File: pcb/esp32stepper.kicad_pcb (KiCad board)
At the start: 4 copper layers, 40 x 40 mm, 86 parts, among them J1 JTAG, J2 Stepper, J3 Display 0.96" 128x96, J4 IO, J5 Qwiic_Vertical, J6 FAN, J7 PWR, J8 USB_C_Receptacle_USB2.0_14P, Q1 IRLML9301, Q2 IRLML9301, SW1 RST, SW3 BOOT, SW4 B1, SW5 B2, U1 TMC2208-LA, U2 ESP32-S3-MINI-1, U3 MPU-9250, U4 AS5048B, U5 LM555xMM, U6 TPS56339DDC, U7 CH224K, U8 BME280

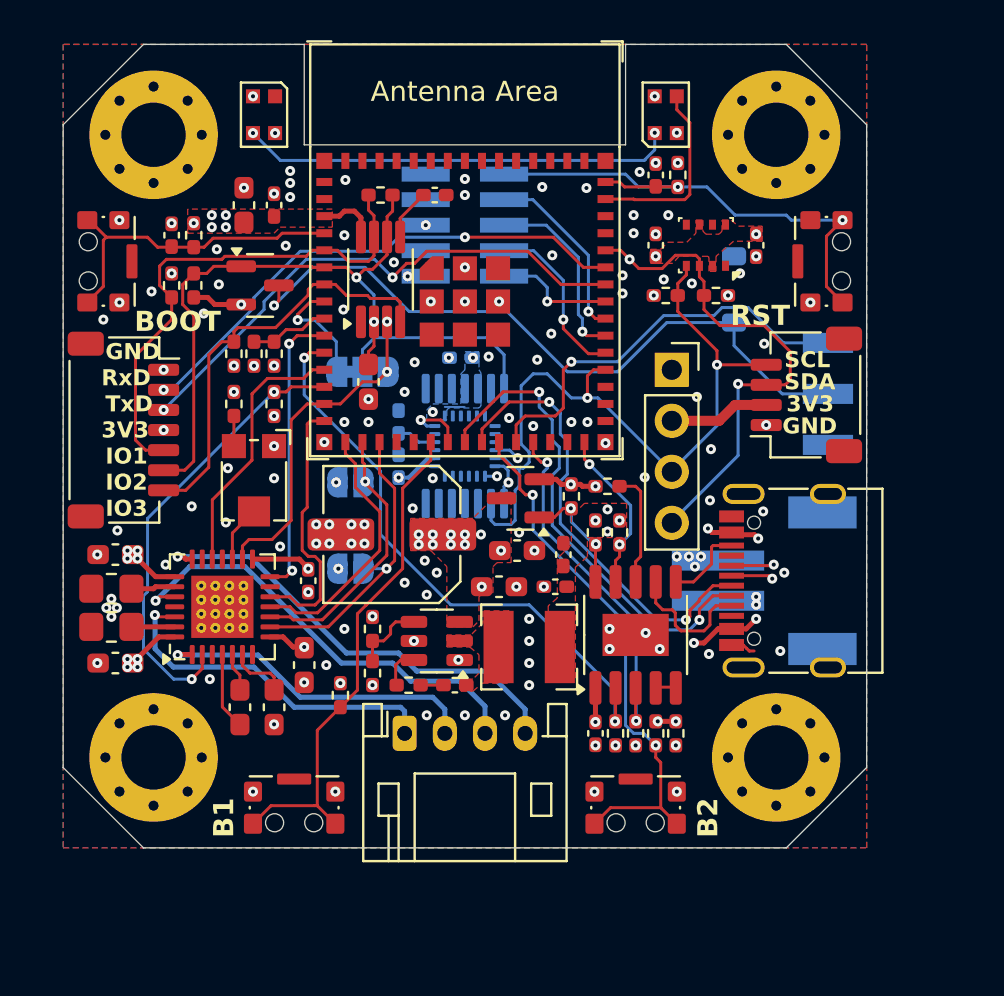
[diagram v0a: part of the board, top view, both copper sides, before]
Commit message: major update to v1.1
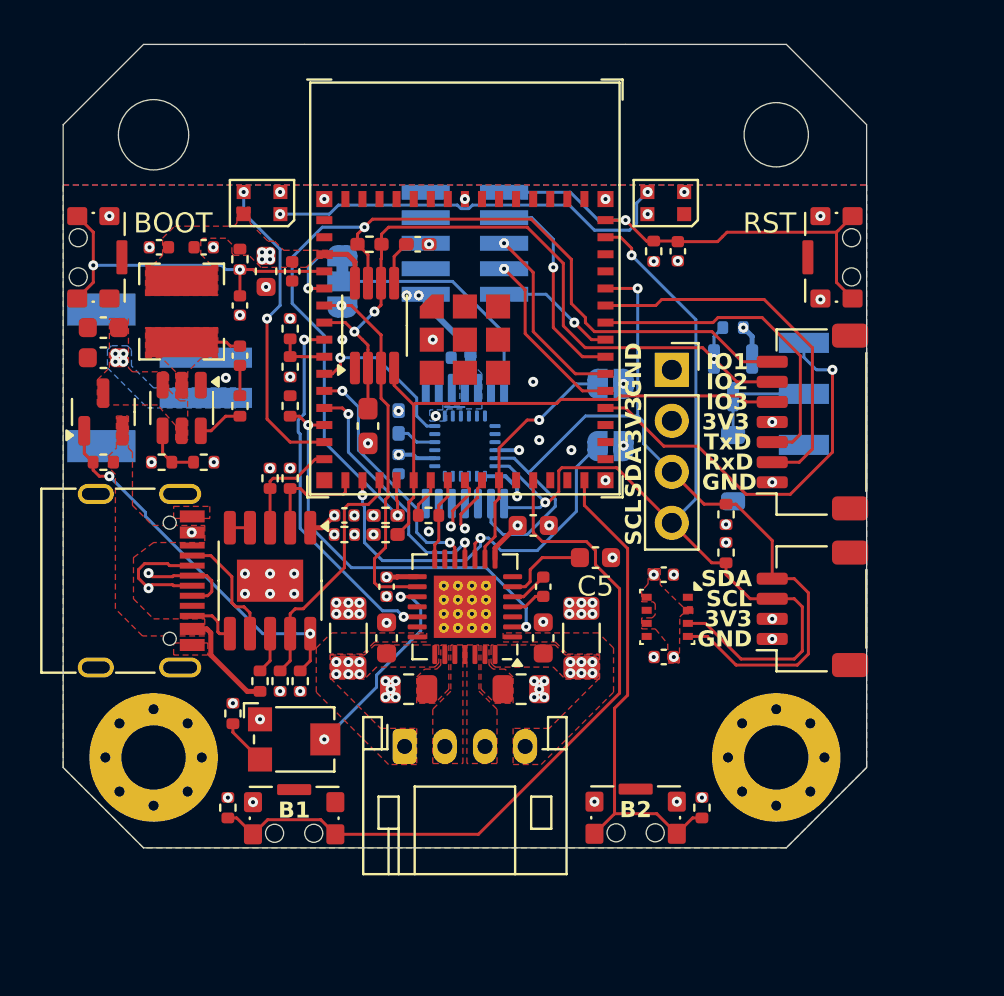
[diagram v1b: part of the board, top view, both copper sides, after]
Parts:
- added C25: 100nF 50V, Capacitor_SMD:C_0603_1608Metric, F.Cu at (86.1, 139.6)
- added R27: 10k, Resistor_SMD:R_0402_1005Metric, F.Cu at (88.2, 133.4)
- C1, C12, C13, C16, C19, C2, C20, C21, C22, C23, C24, C9: footprint Capacitor_SMD:C_0402_1005Metric_Pad0.74x0.62mm_HandSolder -> Capacitor_SMD:C_0402_1005Metric
- C10: value 100µF 35V -> 10µF 50V; footprint Capacitor_SMD:C_Elec_6.3x7.7 -> Capacitor_SMD:C_1206_3216Metric
- C15, C17, C4, C6: footprint Capacitor_SMD:C_0603_1608Metric_Pad1.08x0.95mm_HandSolder -> Capacitor_SMD:C_0603_1608Metric
- C3: footprint Capacitor_SMD:C_0603_1608Metric_Pad1.08x0.95mm_HandSolder -> Capacitor_SMD:C_0402_1005Metric
- C5: value 100nF 35V -> 100nF 50V; footprint Capacitor_SMD:C_0603_1608Metric_Pad1.08x0.95mm_HandSolder -> Capacitor_SMD:C_0603_1608Metric
- C7: value 1µF 35V -> 10µF 50V; footprint Capacitor_SMD:C_0603_1608Metric_Pad1.08x0.95mm_HandSolder -> Capacitor_SMD:C_1206_3216Metric
- C8: value 1µF 35V -> 100nF 50V; footprint Capacitor_SMD:C_0603_1608Metric_Pad1.08x0.95mm_HandSolder -> Capacitor_SMD:C_0603_1608Metric
- H2: footprint MountingHole:MountingHole_3.2mm_M3_Pad_Via -> MountingHole:MountingHole_3.2mm_M3
- H3: footprint MountingHole:MountingHole_3.2mm_M3_Pad_Via -> MountingHole:MountingHole_3.5mm
- Q1: moved to B.Cu
- R1, R10, R11, R13, R17, R18, R19, R2, R20, R21, R22, R23, R24, R25, R26, R3, R4, R5, R8, R9: footprint Resistor_SMD:R_0402_1005Metric_Pad0.72x0.64mm_HandSolder -> Resistor_SMD:R_0402_1005Metric
- R12: footprint Resistor_SMD:R_0402_1005Metric_Pad0.72x0.64mm_HandSolder -> Resistor_SMD:R_0402_1005Metric; moved to B.Cu
- R6, R7: footprint Resistor_SMD:R_0805_2012Metric_Pad1.20x1.40mm_HandSolder -> Resistor_SMD:R_0805_2012Metric
- moved J7 34.4 mm to (73.4, 126.6), turned to -90 degrees
- moved J4 34.3 mm to (107.3, 128.8), turned to 90 degrees
- moved J8 34.3 mm to (72.7, 136.7), turned to -90 degrees
- moved R12 26.9 mm to (103.3, 124.1), turned to 180 degrees
- moved C22 25.3 mm to (74.8, 120.1), turned to 180 degrees
- moved C21 24.3 mm to (77.0, 120.1), turned to 0 degrees
- moved L1 24.0 mm to (75.9, 123.3), turned to 90 degrees
- moved Q1 24.0 mm to (103.3, 126.6), turned to -90 degrees
- moved C17 23.5 mm to (72.0, 124.1), turned to 180 degrees
- moved R22 23.4 mm to (72.0, 130.8), turned to 180 degrees
- moved C7 23.2 mm to (95.8, 139.6), turned to 90 degrees
- moved C15 22.7 mm to (72.0, 125.6), turned to 180 degrees
- moved R23 22.2 mm to (80.3, 131.6), turned to -90 degrees
- moved C8 21.7 mm to (93.9, 139.6), turned to 90 degrees
- moved Q2 21.2 mm to (72.0, 128.3), turned to 90 degrees
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- renumbered D1 to LED1, D2 to LED2
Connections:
- J4 pad 5: /IO1 -> /IO3
- J4 pad 7: /IO3 -> /IO1
- U1 pad 1: Net-(J2-Pin_2) -> Net-(J2-Pin_4)
- U1 pad 21: Net-(J2-Pin_4) -> Net-(J2-Pin_1)
- U1 pad 24: Net-(J2-Pin_3) -> Net-(J2-Pin_2)
- U1 pad 26: Net-(J2-Pin_1) -> Net-(J2-Pin_3)
- U2 pad 10: /PD_UART -> MPU_INT
- U2 pad 11: CFG2 -> INDEX
- U2 pad 12: DIR -> DIAG
- U2 pad 14: STEP -> RGB
- U2 pad 15: INDEX -> CFG3
- U2 pad 16: DIAG -> CFG2
- U2 pad 18: /MS1 -> CFG1
- U2 pad 19: unconnected-(U2-GPIO15/U0RTS/ADC2_CH4/XTAL_32K_P-Pad19) -> /IO1
- U2 pad 20: unconnected-(U2-GPIO16/U0CTS/ADC2_CH5/XTAL_32K_N-Pad20) -> /IO3
- U2 pad 21: BTN1 -> Net-(U2-GPIO17/U1TXD/ADC2_CH6)
- U2 pad 22: MPU_INT -> /PD_UART
- U2 pad 25: BTN2 -> /MS1
- U2 pad 26: /TACHO -> unconnected-(U2-GPIO26-Pad26)
- U2 pad 27: CFG3 -> BTN1
- U2 pad 30: CFG1 -> BTN2
- U2 pad 34: SCL -> /TACHO
- U2 pad 41: SDA -> SCL
- U2 pad 44: RGB -> SDA
- U2 pad 5: /IO1 -> PWM
- U2 pad 6: /IO2 -> STEP
- U2 pad 7: /IO3 -> /IO2
- U2 pad 8: PWM -> DIR
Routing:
- net Net-(D3-K): track 34.8 -> 5.44 mm, vias 1 -> 0
- net CFG2: track 29.6 -> 5.46 mm, vias 2 -> 0
- net /IO1: track 26.1 -> 48.8 mm, vias 0 -> 2
- net Net-(J2-Pin_4): track 22.4 -> 0.00 mm, vias 1 -> 0
- net Net-(J2-Pin_3): track 22.4 -> 0.00 mm, vias 1 -> 0
- net Net-(J2-Pin_1): track 17.5 -> 0.00 mm, vias 1 -> 0
- net Net-(J2-Pin_2): track 16.4 -> 0.00 mm, vias 1 -> 0
- net CFG3: track 18.0 -> 5.47 mm, vias 2 -> 0
- net /PG: track 6.00 -> 18.5 mm
- net BTN1: track 25.3 -> 37.0 mm
- net SDA: track 37.3 -> 48.7 mm, vias 3 -> 2
- net /TXD: track 27.3 -> 16.1 mm, vias 2 -> 0
- net /PD_UART: track 14.5 -> 4.19 mm, vias 2 -> 0
- net SCL: track 37.4 -> 47.5 mm, vias 2 -> 1
- net /IO2: track 29.5 -> 37.6 mm, vias 2 -> 3
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- added copper zone on F.Cu, net Net-(J2-Pin_1)
- added copper zone on F.Cu, net Net-(J2-Pin_2)
- added copper zone on F.Cu, net Net-(J2-Pin_3)
- added copper zone on F.Cu, net Net-(J2-Pin_4)
- added copper zone on F.Cu, net Net-(U1-BRA)
- added copper zone on F.Cu, net Net-(U1-BRB)
- added copper zone on F.Cu, net VBUS
- added copper zone on B.Cu, net VDD
- removed copper zone on In2.Cu, net VBUS
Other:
- outline, holes or cut-outs redrawn
- board text added: "(bottom)"
- board text added: "USB-C Connector"
- board text added: "alt. Power Connector"
- board text removed: "USB-C Connector (top)"
- board text removed: "VDD"
- board text removed: "external Power Connector (bottom)"
